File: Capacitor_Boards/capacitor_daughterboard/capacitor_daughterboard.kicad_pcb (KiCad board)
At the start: 2 copper layers, 19 x 20 mm, 3 parts, among them J1 Conn_01x05, J2 Conn_01x05

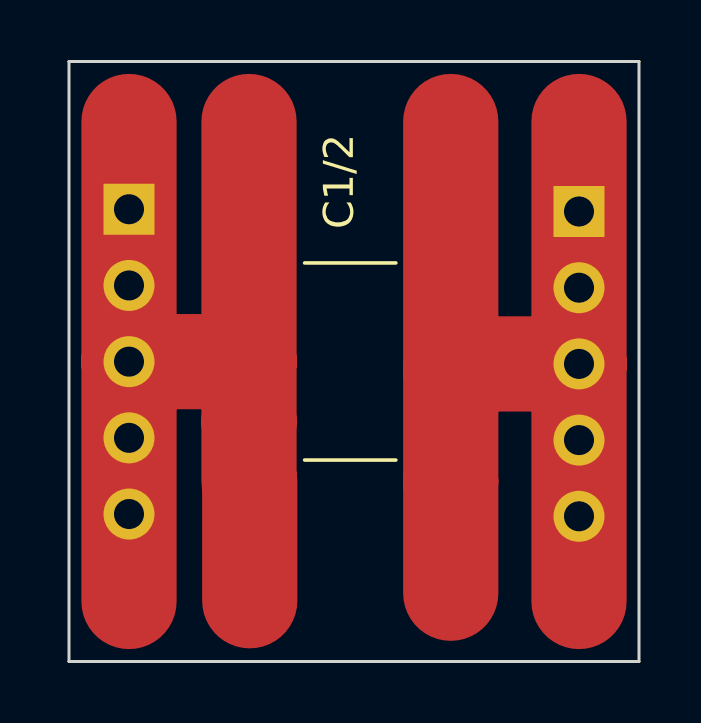
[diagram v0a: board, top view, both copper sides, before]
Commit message: Finalized boards
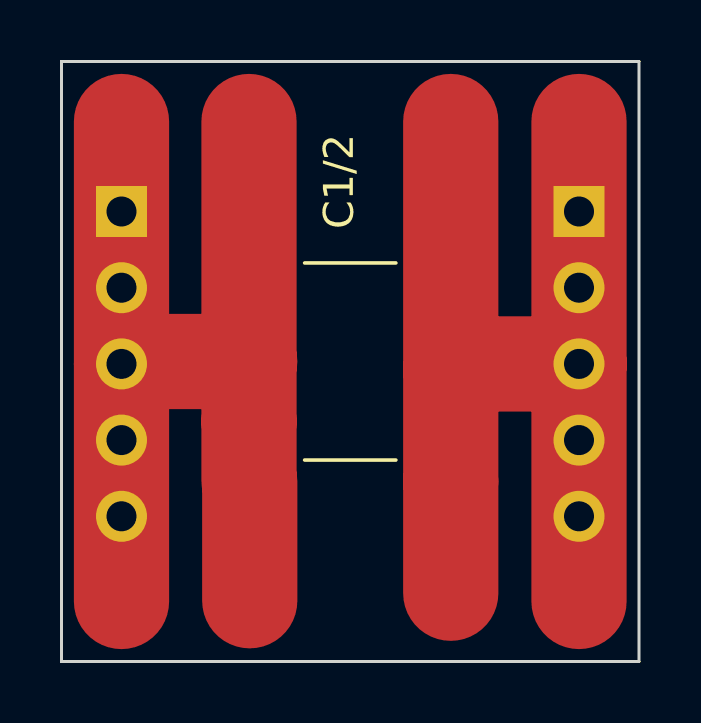
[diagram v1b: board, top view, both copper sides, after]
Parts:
- moved J1 0.26 mm to (132.8, 76.0)
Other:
- board size 19 x 20 mm -> 19.2 x 20 mm
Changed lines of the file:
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@@
   )
   (footprint "Connector_PinHeader_2.54mm:PinHeader_1x05_P2.54mm_Vertical" (layer "B.Cu")
-    (at 133 75.925 180)
+    (at 132.75 76 180)
     (descr "Through hole straight pin header, 1x05, 2.54mm pitch, single row")
     (tags "Through hole pin header THT 1x05 2.54mm single row")
@@
     )
   )
-  (gr_rect (start 131 71) (end 150 91) (layer "Edge.Cuts") (width 0.1) (fill none))
+  (gr_rect (start 130.75 71) (end 150 91) (layer "Edge.Cuts") (width 0.1) (fill none))
   (segment (start 148 81.08) (end 143.92 81.08) (width 3.175) (layer "F.Cu") (net 1))
   (segment (start 143.92 81.08) (end 143.725 81.275) (width 3.175) (layer "F.Cu") (net 1))
@@
   (segment (start 148 81.08) (end 148 89) (width 3.175) (layer "F.Cu") (net 1))
   (segment (start 137 73) (end 137 81) (width 3.175) (layer "F.Cu") (net 2))
-  (segment (start 133 81.005) (end 133 89) (width 3.175) (layer "F.Cu") (net 2))
+  (segment (start 132.83 81) (end 132.75 81.08) (width 3.175) (layer "F.Cu") (net 2))
   (segment (start 137 83) (end 137 84.975) (width 3.175) (layer "F.Cu") (net 2))
   (segment (start 137 81) (end 137 83) (width 3.175) (layer "F.Cu") (net 2))
   (segment (start 137 81) (end 136.995 81.005) (width 3.175) (layer "F.Cu") (net 2))
-  (segment (start 136.995 81.005) (end 133 81.005) (width 3.175) (layer "F.Cu") (net 2))
-  (segment (start 133 73) (end 133 81.005) (width 3.175) (layer "F.Cu") (net 2))
+  (segment (start 132.75 81.08) (end 132.75 89) (width 3.175) (layer "F.Cu") (net 2))
+  (segment (start 132.75 81.08) (end 132.75 73) (width 3.175) (layer "F.Cu") (net 2))
   (segment (start 137.025 85) (end 137.025 88.975) (width 3.175) (layer "F.Cu") (net 2))
+  (segment (start 137.025 81) (end 132.83 81) (width 3.175) (layer "F.Cu") (net 2))
 )
